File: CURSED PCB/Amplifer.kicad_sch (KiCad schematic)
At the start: 11 parts, among them U1 MCP3562-E_ST, U2 OPA196xDBV, U3 MCP1501-30xSN

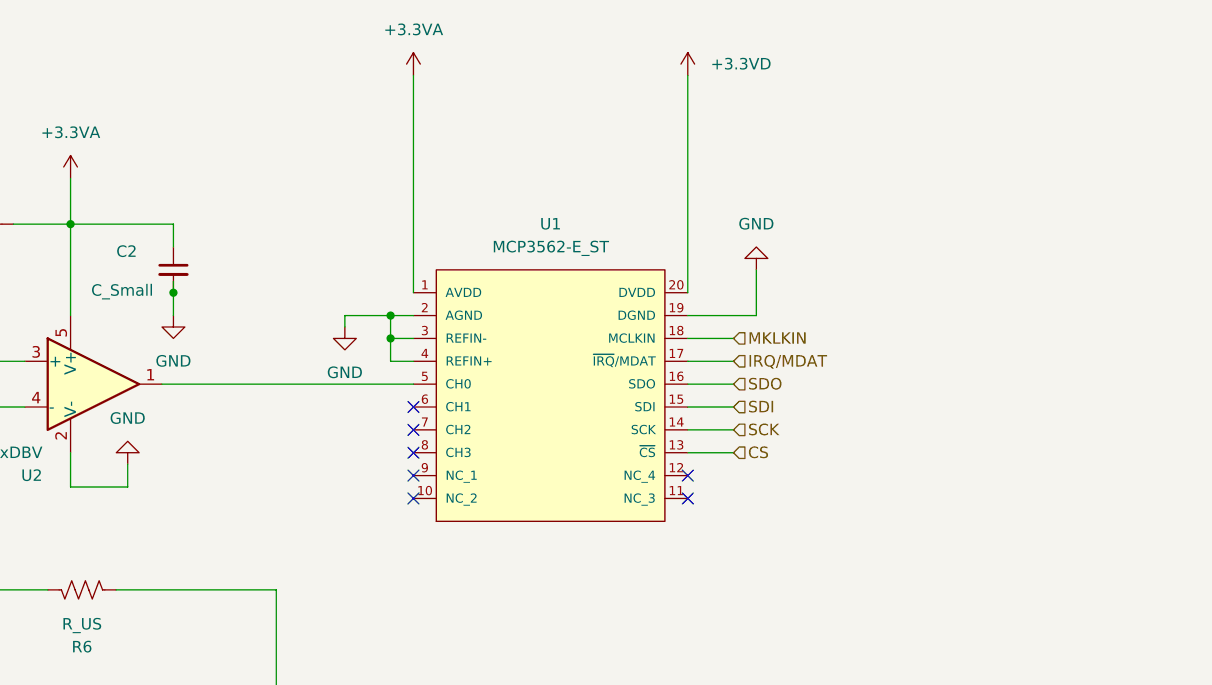
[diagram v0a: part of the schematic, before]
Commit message: Added some amplifer stuff
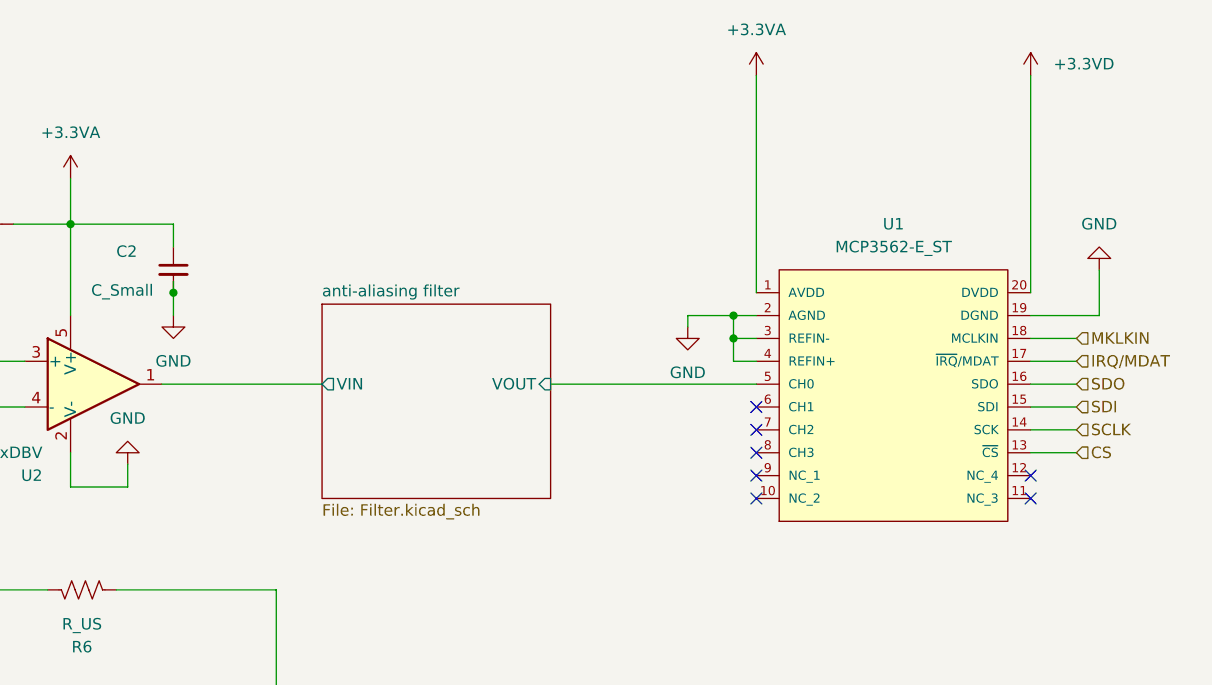
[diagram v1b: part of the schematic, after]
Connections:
- net anti-aliasing filter/VIN: now reaches U2.1
- net anti-aliasing filter/VIN: no longer U1.5 (CH0)
- net SCK renamed SCLK
- new net anti-aliasing filter/VOUT: U1.5 (CH0)
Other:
- added sheet anti-aliasing filter (Filter.kicad_sch)
- moved on the sheet: U1
